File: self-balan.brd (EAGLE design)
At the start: 160 x 100 mm, 15 parts, among them U1 ATMEGA328P_TQFP

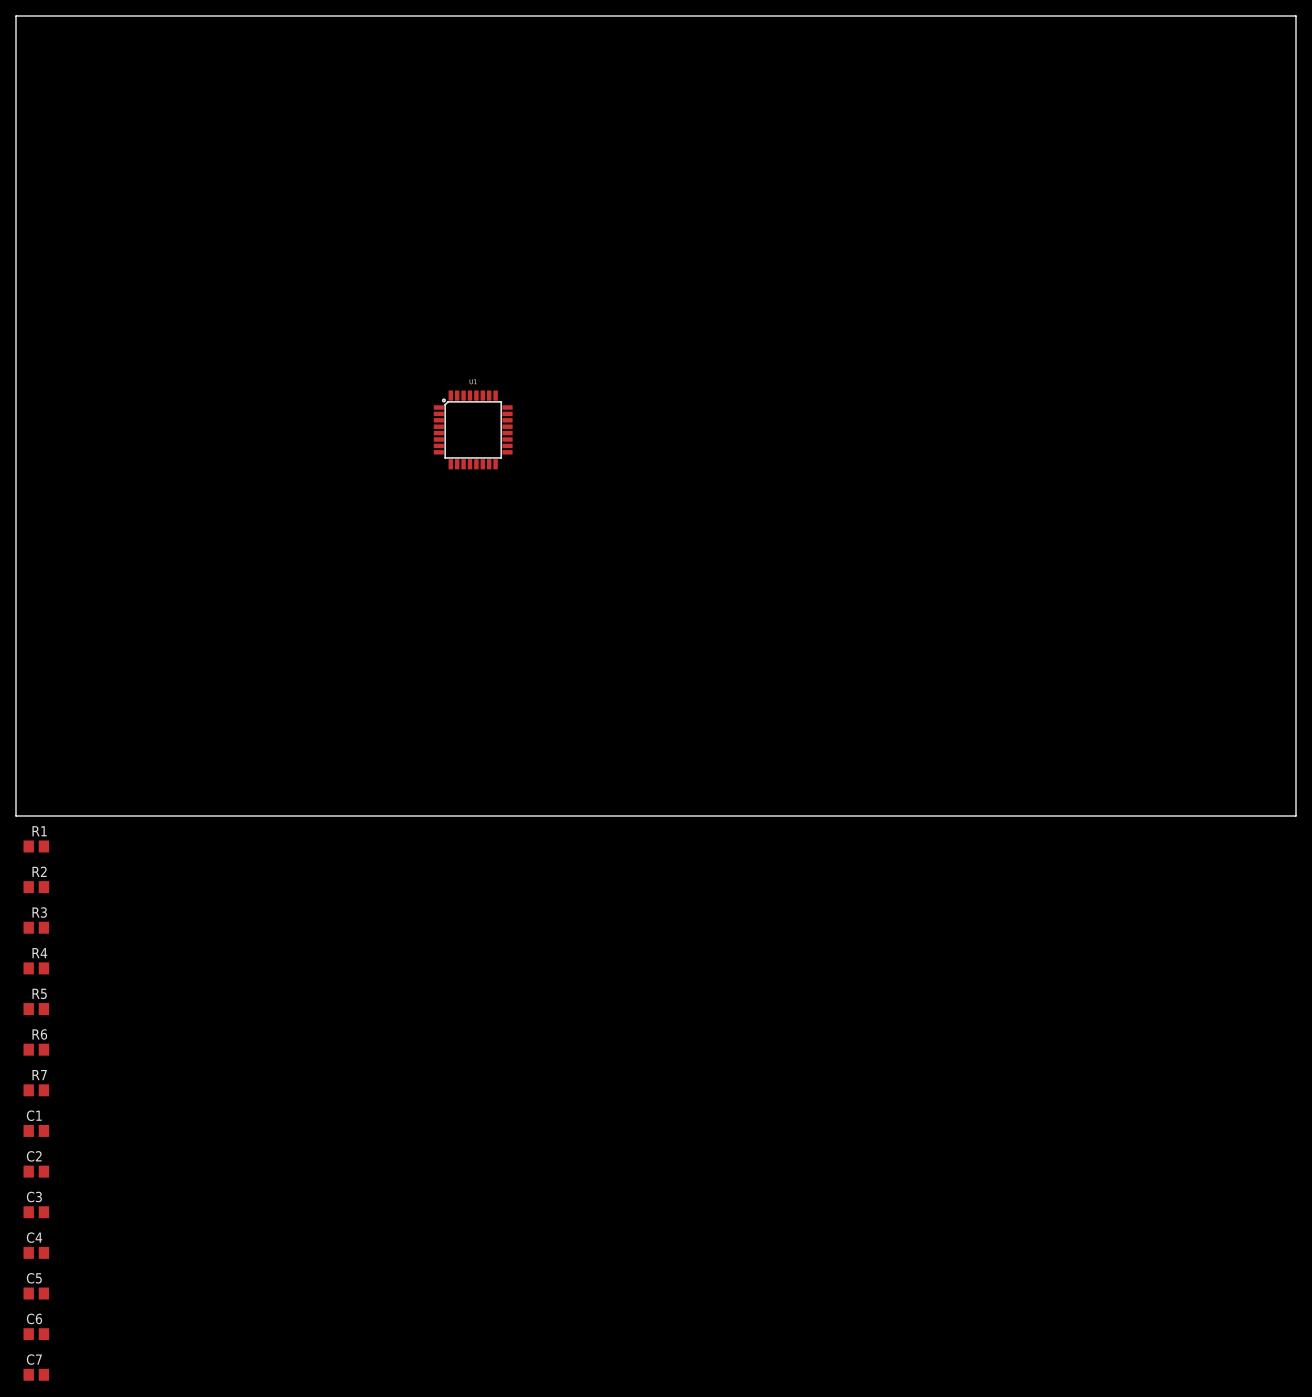
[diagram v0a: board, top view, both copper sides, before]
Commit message: Minor fix
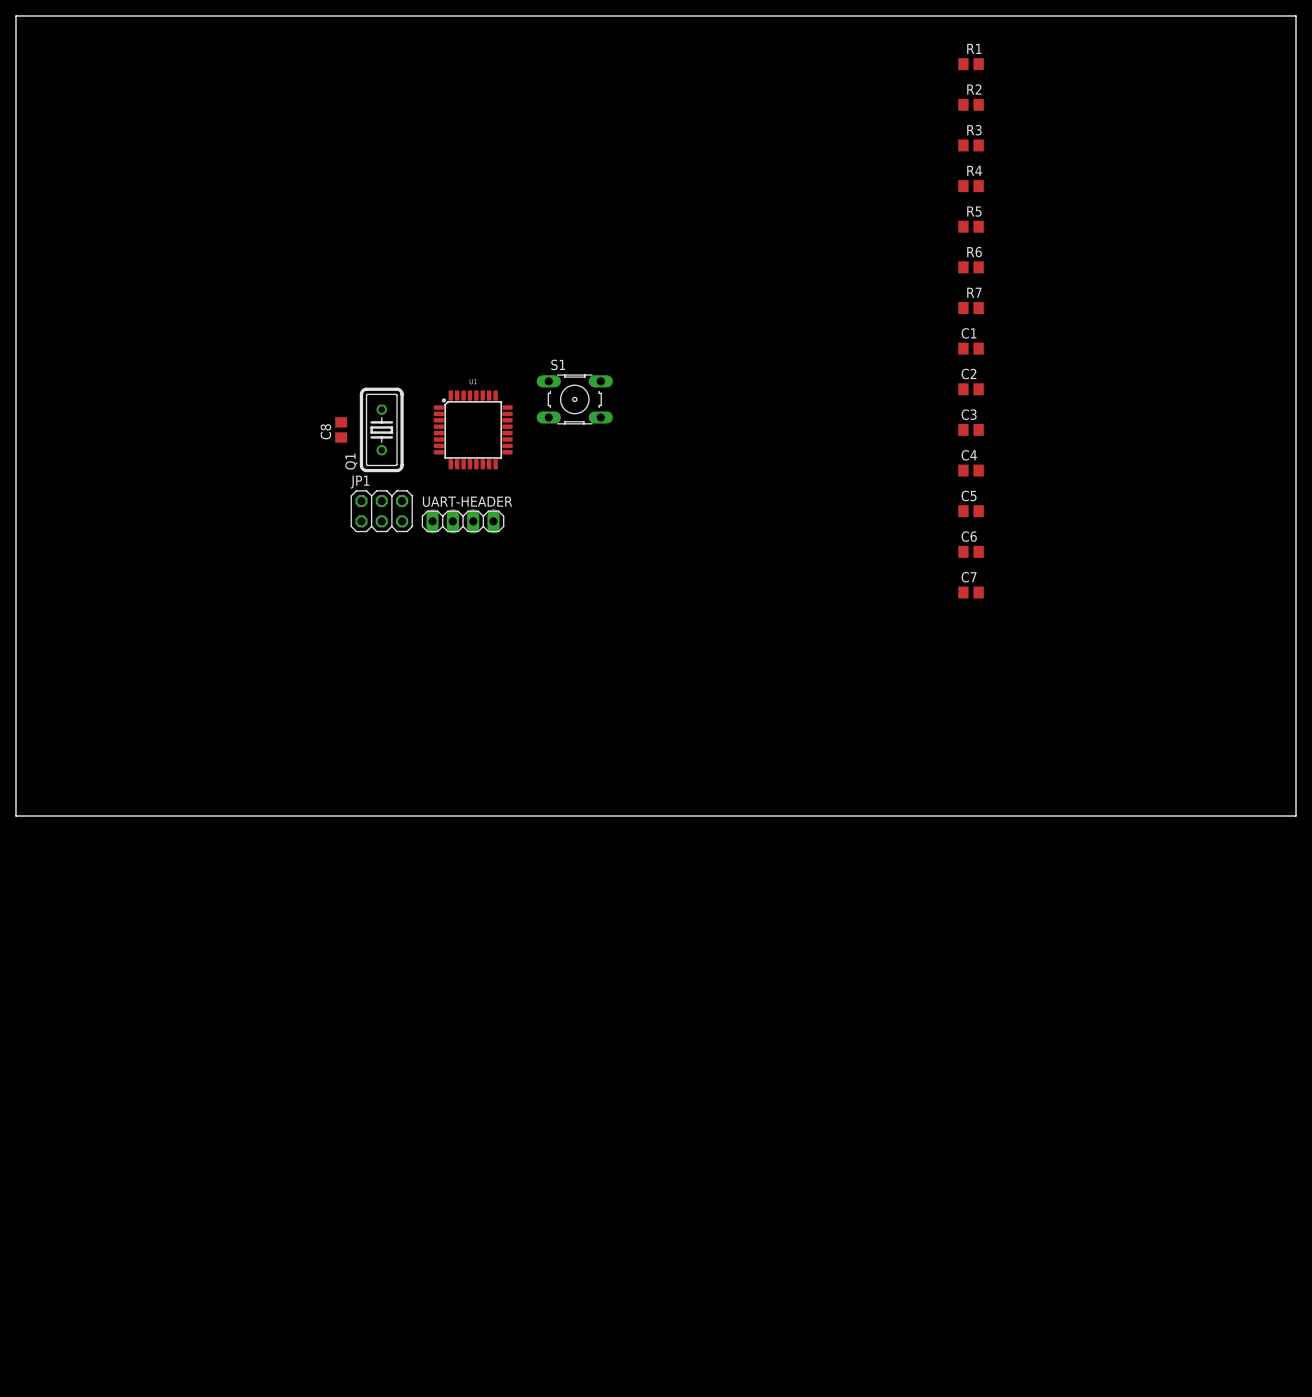
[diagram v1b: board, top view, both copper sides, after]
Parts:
- added C8: (no value), rcl:C0805
- added JP1: (no value), pinhead:2X03
- added Q1: (no value), adafruit:HC18U-V
- added S1: (no value), switch-omron:B3F-10XX
- added UART-HEADER: (no value), pinhead:1X04
- moved C1 152.4 mm to (119.4, 58.4)
- moved C2 152.4 mm to (119.4, 53.3)
- moved C3 152.4 mm to (119.4, 48.3)
- moved C4 152.4 mm to (119.4, 43.2)
- moved C5 152.4 mm to (119.4, 38.1)
- moved C6 152.4 mm to (119.4, 33.0)
- moved C7 152.4 mm to (119.4, 27.9)
- moved R1 152.4 mm to (119.4, 94.0)
- moved R2 152.4 mm to (119.4, 88.9)
- moved R3 152.4 mm to (119.4, 83.8)
- moved R4 152.4 mm to (119.4, 78.7)
- moved R5 152.4 mm to (119.4, 73.7)
- moved R6 152.4 mm to (119.4, 68.6)
- moved R7 152.4 mm to (119.4, 63.5)
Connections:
- new net +5V: R3.2
- new net GND: C2.1, C2.2, C8.2, JP1.6, Q1.2, S1.3, S1.4, U1.7, UART-HEADER.4
- new net MISO: JP1.1, U1.16
- new net MOSI: JP1.4, U1.15
- new net N$3: C3.2, U1.21, U1.3, U1.5
- new net N$4: C8.1, Q1.1, U1.8
- new net RST: JP1.5, R3.1, S1.1, S1.2, U1.29
- new net RXD: U1.31, UART-HEADER.2
- new net SCK: JP1.3, U1.17
- new net TXD: U1.30, UART-HEADER.1
- new net VCC: C3.1, JP1.2, U1.18, U1.20, U1.4, U1.6, UART-HEADER.3
